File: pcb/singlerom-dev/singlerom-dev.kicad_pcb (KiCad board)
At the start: 2 copper layers, 96.3 x 48.2 mm, 28 parts, among them J4 PWR Breakout, U2 MX29LV320EBTI-70G

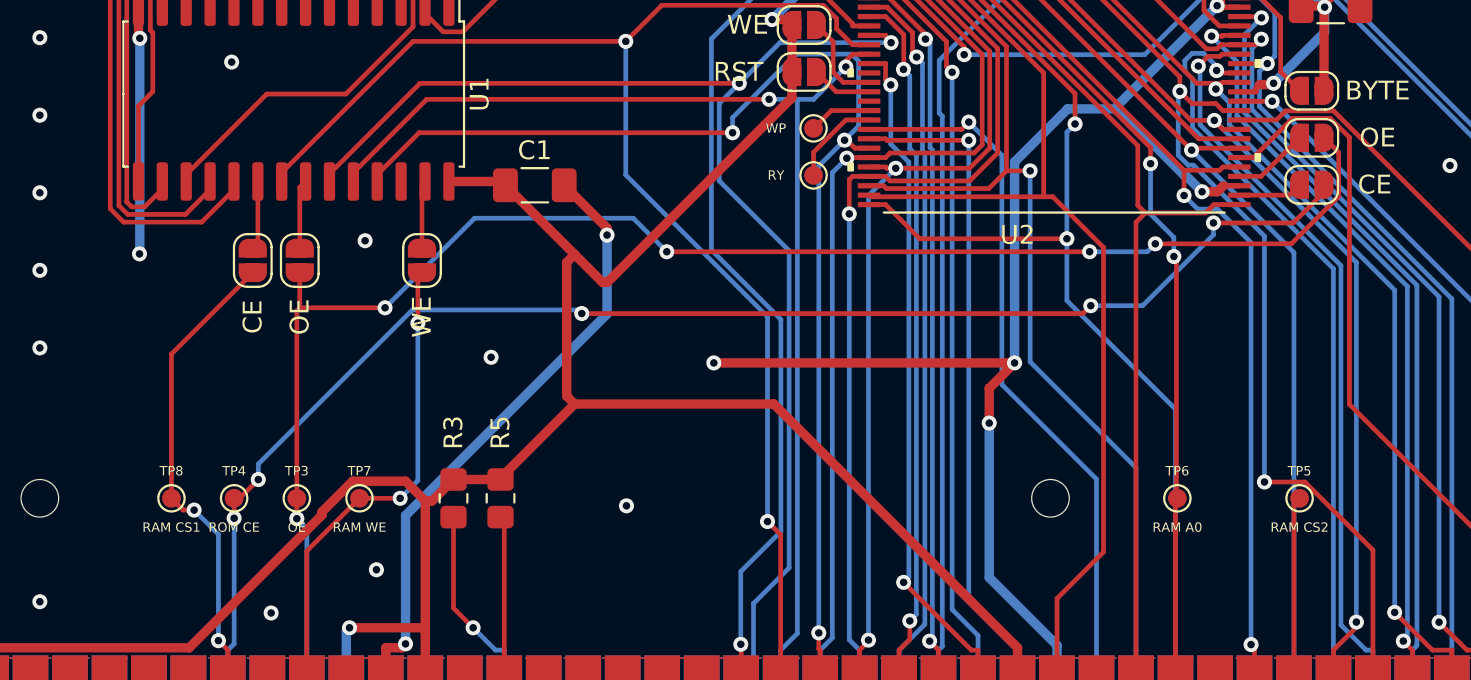
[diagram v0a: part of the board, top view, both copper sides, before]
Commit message: tweaks
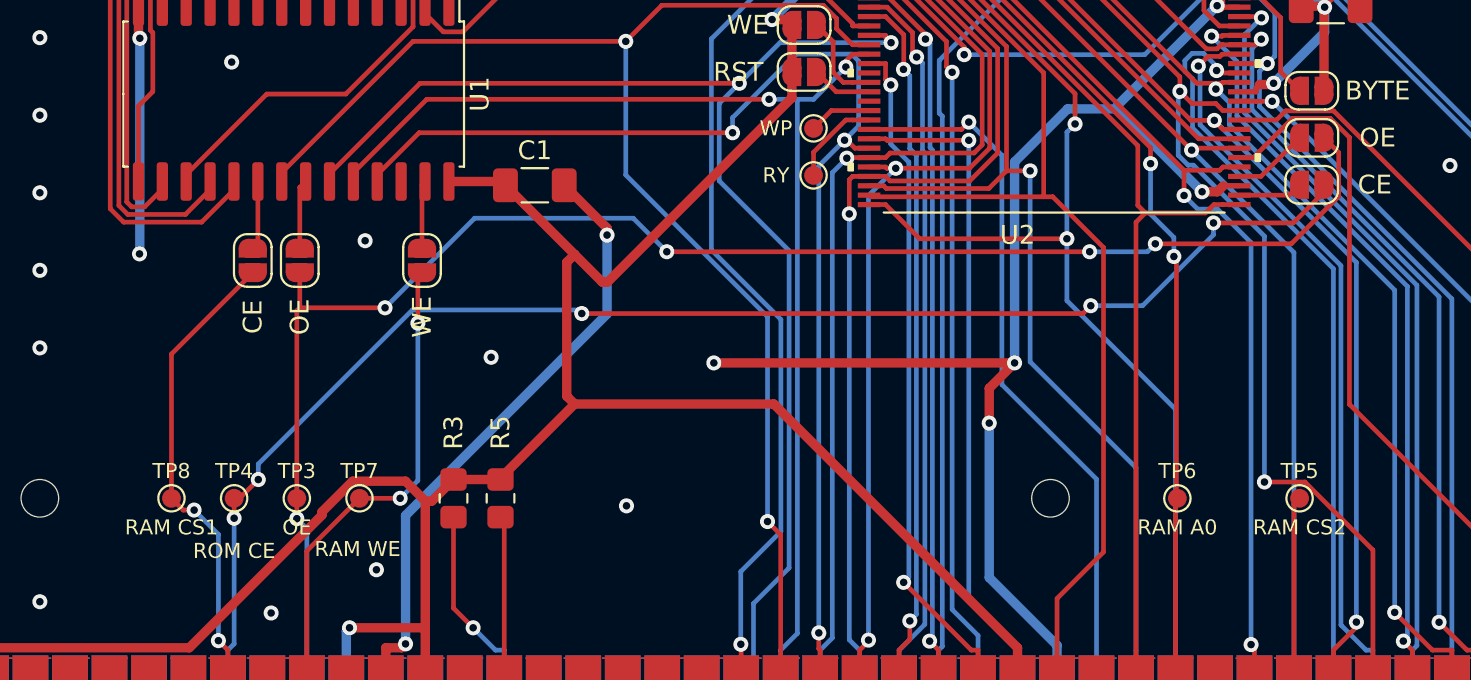
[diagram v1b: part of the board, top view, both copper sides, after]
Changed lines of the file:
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@@
     )
     (fp_text value "RY" (at -2 0) (layer "F.SilkS")
-        (effects (font (size 0.5 0.5) (thickness 0.1)))
+        (effects (font (size 0.8 0.8) (thickness 0.1)))
     )
     (fp_text user "${REFERENCE}" (at 0 -1.45) (layer "F.Fab") hide
@@
     )
     (fp_text value "WP" (at -2 0) (layer "F.SilkS")
-        (effects (font (size 0.5 0.5) (thickness 0.1)))
+        (effects (font (size 0.8 0.8) (thickness 0.1)))
     )
     (fp_text user "${REFERENCE}" (at 0 -1.45) (layer "F.Fab")
@@
     (attr exclude_from_pos_files)
     (fp_text reference "TP4" (at 0 -1.448) (layer "F.SilkS")
-        (effects (font (size 0.5 0.5) (thickness 0.1)))
-    )
-    (fp_text value "ROM CE" (at 0 1.55) (layer "F.SilkS")
-        (effects (font (size 0.5 0.5) (thickness 0.1)))
+        (effects (font (size 0.8 0.8) (thickness 0.1)))
+    )
+    (fp_text value "ROM CE" (at 0 2.8) (layer "F.SilkS")
+        (effects (font (size 0.8 0.8) (thickness 0.1)))
     )
     (fp_text user "${REFERENCE}" (at 0 -1.45) (layer "F.Fab")
@@
     (attr exclude_from_pos_files)
     (fp_text reference "TP3" (at 0 -1.448) (layer "F.SilkS")
-        (effects (font (size 0.5 0.5) (thickness 0.1)))
+        (effects (font (size 0.8 0.8) (thickness 0.1)))
     )
     (fp_text value "OE" (at 0 1.55) (layer "F.SilkS")
-        (effects (font (size 0.5 0.5) (thickness 0.1)))
+        (effects (font (size 0.8 0.8) (thickness 0.1)))
     )
     (fp_text user "${REFERENCE}" (at 0 -1.45) (layer "F.Fab")
@@
     (attr exclude_from_pos_files)
     (fp_text reference "TP7" (at 0 -1.448) (layer "F.SilkS")
-        (effects (font (size 0.5 0.5) (thickness 0.1)))
-    )
-    (fp_text value "RAM WE" (at 0 1.55) (layer "F.SilkS")
-        (effects (font (size 0.5 0.5) (thickness 0.1)))
+        (effects (font (size 0.8 0.8) (thickness 0.1)))
+    )
+    (fp_text value "RAM WE" (at -0.1 2.7) (layer "F.SilkS")
+        (effects (font (size 0.8 0.8) (thickness 0.1)))
     )
     (fp_text user "${REFERENCE}" (at 0 -1.45) (layer "F.Fab")
@@
     (attr exclude_from_pos_files)
     (fp_text reference "TP5" (at 0 -1.448) (layer "F.SilkS")
-        (effects (font (size 0.5 0.5) (thickness 0.1)))
+        (effects (font (size 0.8 0.8) (thickness 0.1)))
     )
     (fp_text value "RAM CS2" (at 0 1.55) (layer "F.SilkS")
-        (effects (font (size 0.5 0.5) (thickness 0.1)))
+        (effects (font (size 0.8 0.8) (thickness 0.1)))
     )
     (fp_text user "${REFERENCE}" (at 0 -1.45) (layer "F.Fab")
@@
     (attr exclude_from_pos_files)
     (fp_text reference "TP6" (at 0 -1.448) (layer "F.SilkS")
-        (effects (font (size 0.5 0.5) (thickness 0.1)))
+        (effects (font (size 0.8 0.8) (thickness 0.1)))
     )
     (fp_text value "RAM A0" (at 0 1.55) (layer "F.SilkS")
-        (effects (font (size 0.5 0.5) (thickness 0.1)))
+        (effects (font (size 0.8 0.8) (thickness 0.1)))
     )
     (fp_text user "${REFERENCE}" (at 0 -1.45) (layer "F.Fab")
@@
     (attr exclude_from_pos_files)
     (fp_text reference "TP8" (at 0 -1.448) (layer "F.SilkS")
-        (effects (font (size 0.5 0.5) (thickness 0.1)))
+        (effects (font (size 0.8 0.8) (thickness 0.1)))
     )
     (fp_text value "RAM CS1" (at 0 1.55) (layer "F.SilkS")
-        (effects (font (size 0.5 0.5) (thickness 0.1)))
+        (effects (font (size 0.8 0.8) (thickness 0.1)))
     )
     (fp_text user "${REFERENCE}" (at 0 -1.45) (layer "F.Fab")
@@
     )
   )
+  (gr_rect (start 101.3 129.7) (end 199 135.5)
+    (stroke (width 0.15) (type solid)) (fill solid) (layer "B.Mask"))
+  (gr_rect (start 101.3 129.7) (end 199 135.5)
+    (stroke (width 0.15) (type solid)) (fill solid) (layer "F.Mask"))
   (gr_line (start 101.75 111.5) (end 101.75 119.25)
     (stroke (width 0.1) (type default)) (layer "Edge.Cuts"))
